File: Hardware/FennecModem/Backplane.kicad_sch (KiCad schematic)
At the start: 28 parts, among them J1 SEL_ADDR, J3 EN_ADDR, J4 CARD_EN_BYPASS, Q901 MMBT3904, U2 SN74CBTLV3245A, U9 LM2596S-5

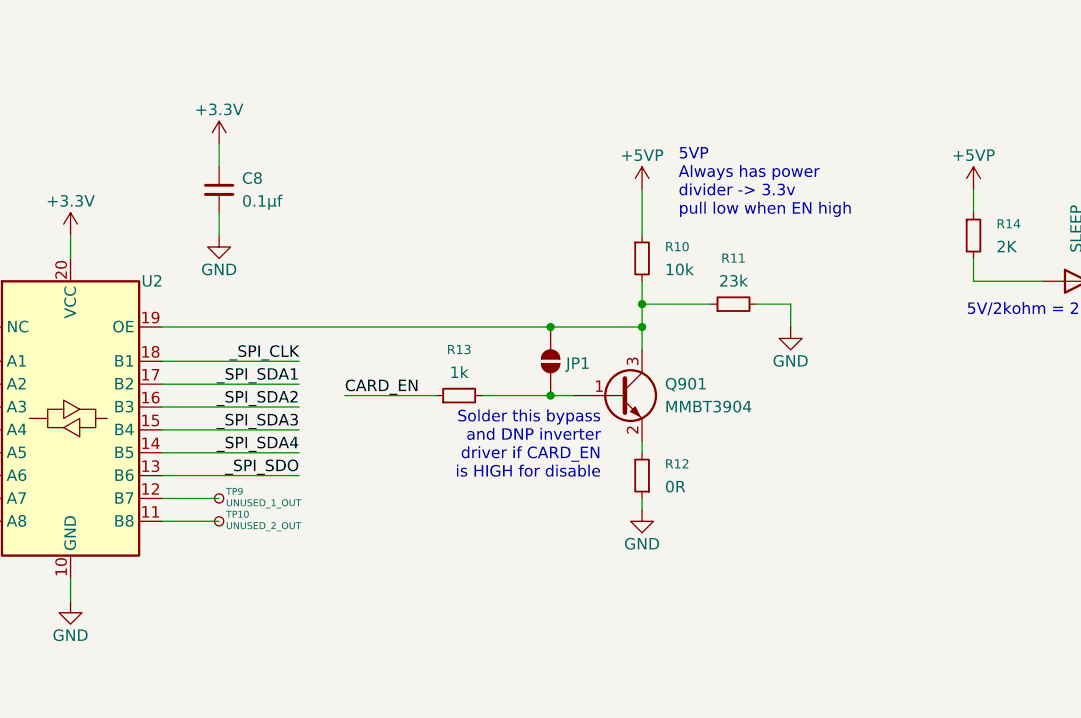
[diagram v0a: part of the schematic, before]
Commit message: Implement suggestions from KA2
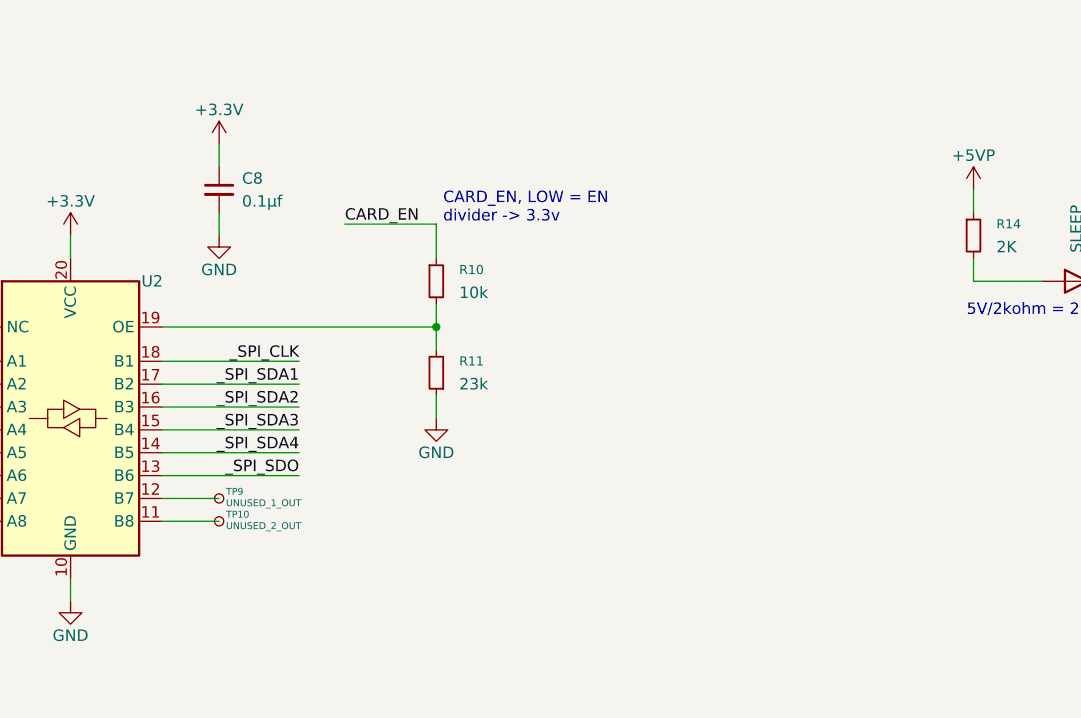
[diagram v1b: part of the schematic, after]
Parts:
- removed JP1: SolderJumper_2_Open, Jumper:SolderJumper-2_P1.3mm_Open_TrianglePad1.0x1.5mm, symbol Jumper:SolderJumper_2_Open
- removed Q901: MMBT3904, Package_TO_SOT_SMD:SOT-23, symbol Transistor_BJT:MMBT3904
- removed R12: 0R, Resistor_SMD:R_0805_2012Metric, symbol Device:R_Small
- removed R13: 1k, Resistor_SMD:R_0805_2012Metric, symbol Device:R_Small
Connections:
- net +5VP: no longer R10.1
- net CARD_EN: now also R10.1
- net GND: now also R11.1; no longer R11.2
- net at R10.2, U2.19 (OE): now also R11.2; no longer R11.1
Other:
- note added: "CARD_EN, LOW = EN divider -> 3.3v"
- note removed: "5VP Always has power divider -> 3.3v pull low when EN high"
- note removed: "Solder this bypass and DNP inverter driver if CARD_EN is HIGH for disable"
- moved on the sheet: R10, R11
